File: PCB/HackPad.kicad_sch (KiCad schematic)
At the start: 10 parts, among them SW1 RotaryEncoder_Switch, SW2 RotaryEncoder_Switch, SW4 SW_Push, SW5 SW_Push, SW6 SW_Push, SW7 SW_Push, U1 Seeed Studio XIAO SAMD21, U2 PCF8574A

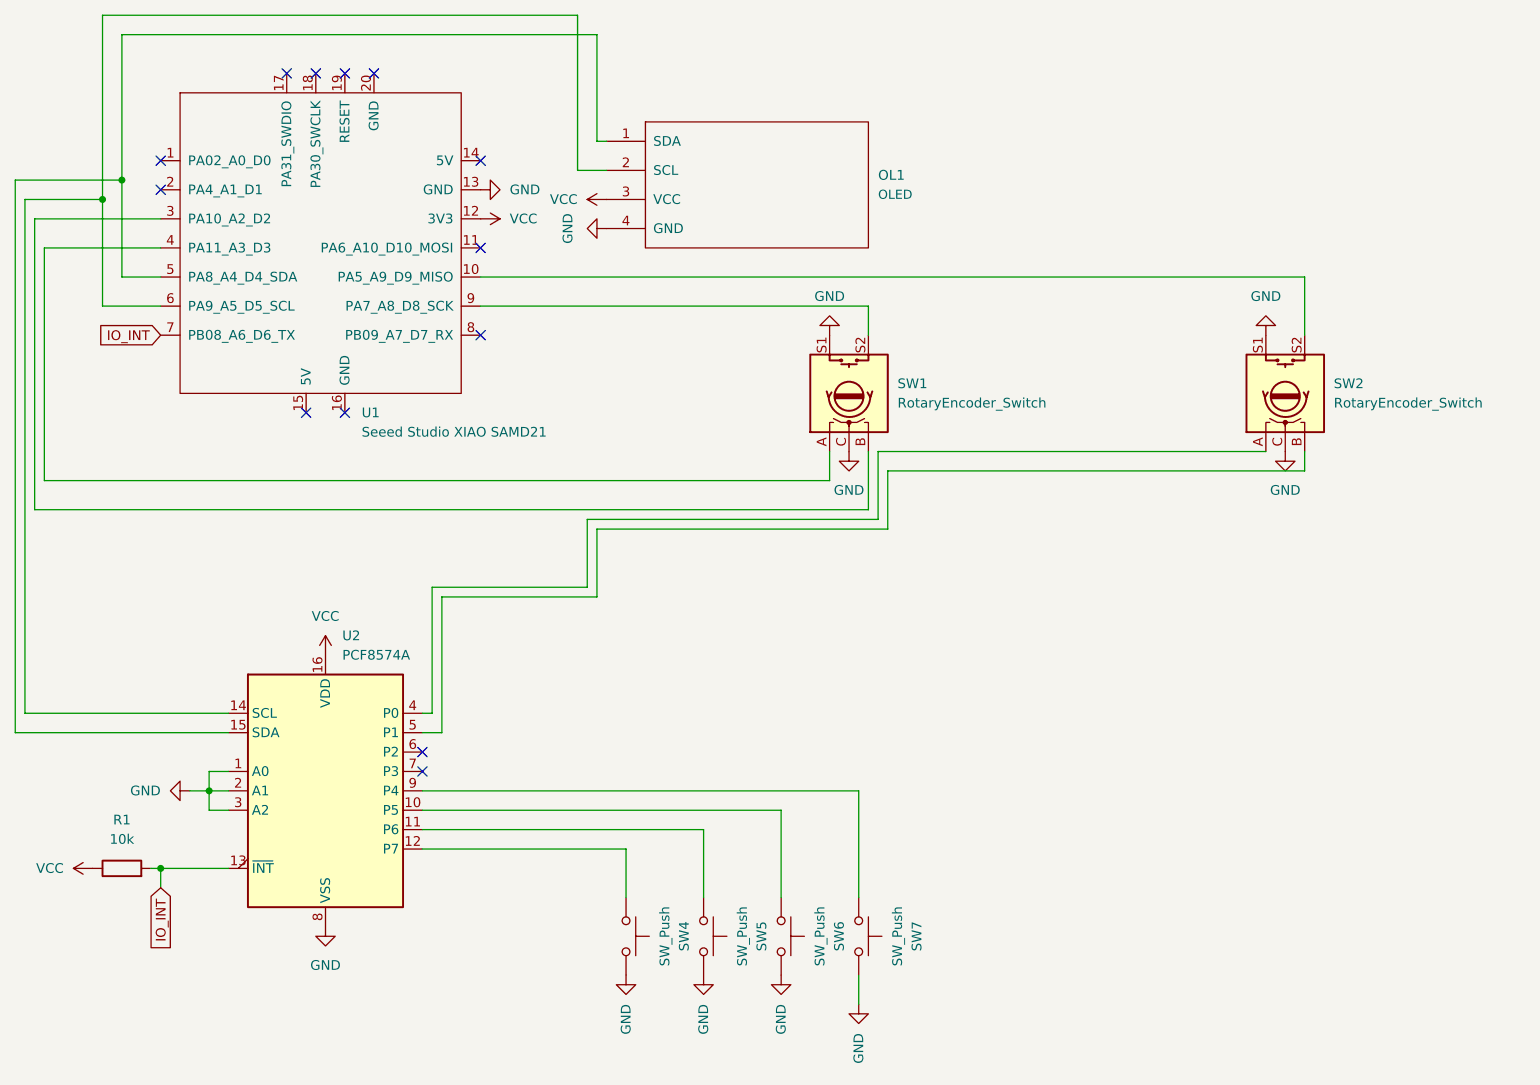
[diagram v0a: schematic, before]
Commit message: Add files via upload
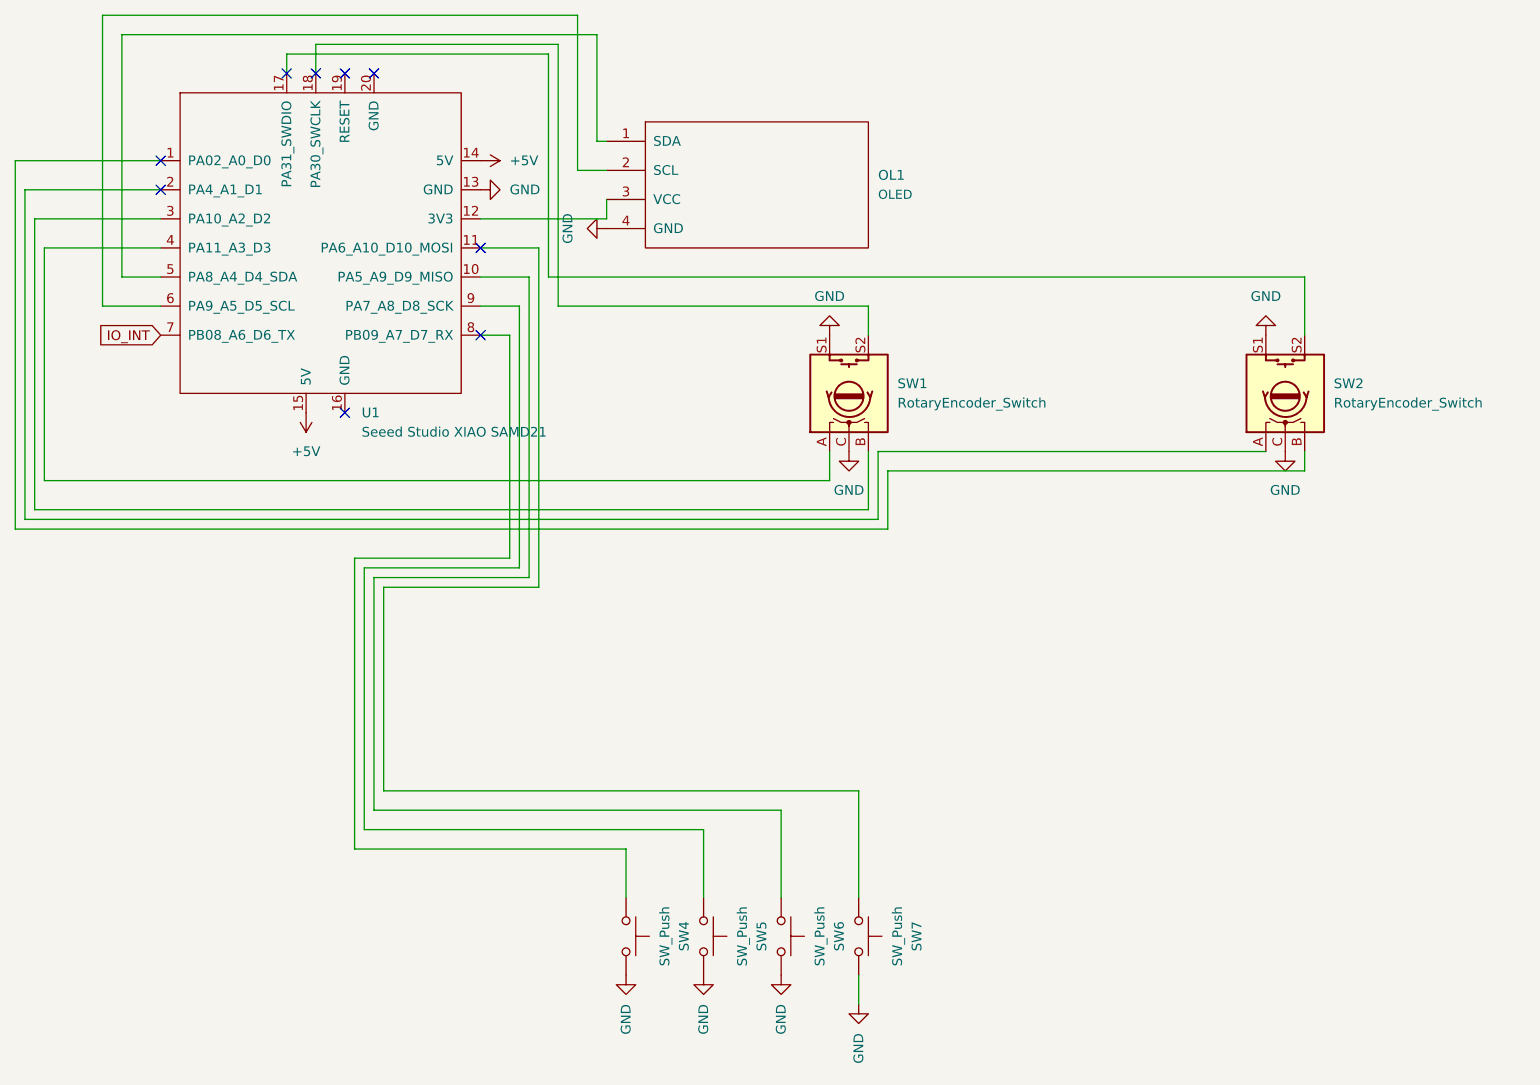
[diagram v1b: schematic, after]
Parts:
- removed R1: 10k, Resistor_THT:R_Axial_DIN0207_L6.3mm_D2.5mm_P10.16mm_Horizontal, symbol Device:R
- removed U2: PCF8574A, Package_DIP:DIP-16_W7.62mm, symbol Interface_Expansion:PCF8574A
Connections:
- net at SW1.S2: now also U1.18 (PA30_SWCLK); no longer U1.9 (PA7_A8_D8_SCK)
- net at SW7.1: now also U1.11 (PA6_A10_D10_MOSI)
- net at SW5.1: now also U1.9 (PA7_A8_D8_SCK)
- net at U1.1 (PA02_A0_D0): now also SW2.B
- net at U1.10 (PA5_A9_D9_MISO): now also SW6.1; no longer SW2.S2
- net +5V: now reaches U1.14 (5V)
- net +5V: now also U1.15 (5V)
- net at U1.17 (PA31_SWDIO): now also SW2.S2
- net at U1.2 (PA4_A1_D1): now also SW2.A
- net at U1.8 (PB09_A7_D7_RX): now also SW4.1
- net VCC: no longer names the net of OL1.3 (VCC), U1.12 (3V3)
- no-connect marks 13 -> 9
